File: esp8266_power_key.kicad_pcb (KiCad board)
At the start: 2 copper layers, 25 parts, among them P1 CONN_01X06, P2 CONN_01X06, Q1 Q_PMOS_GDS, Q2 Q_PMOS_GDS, Q3 BC849, Q4 BC849, U1 ESP-01v090, U2 LP2988AIMX-3.3/NOPB

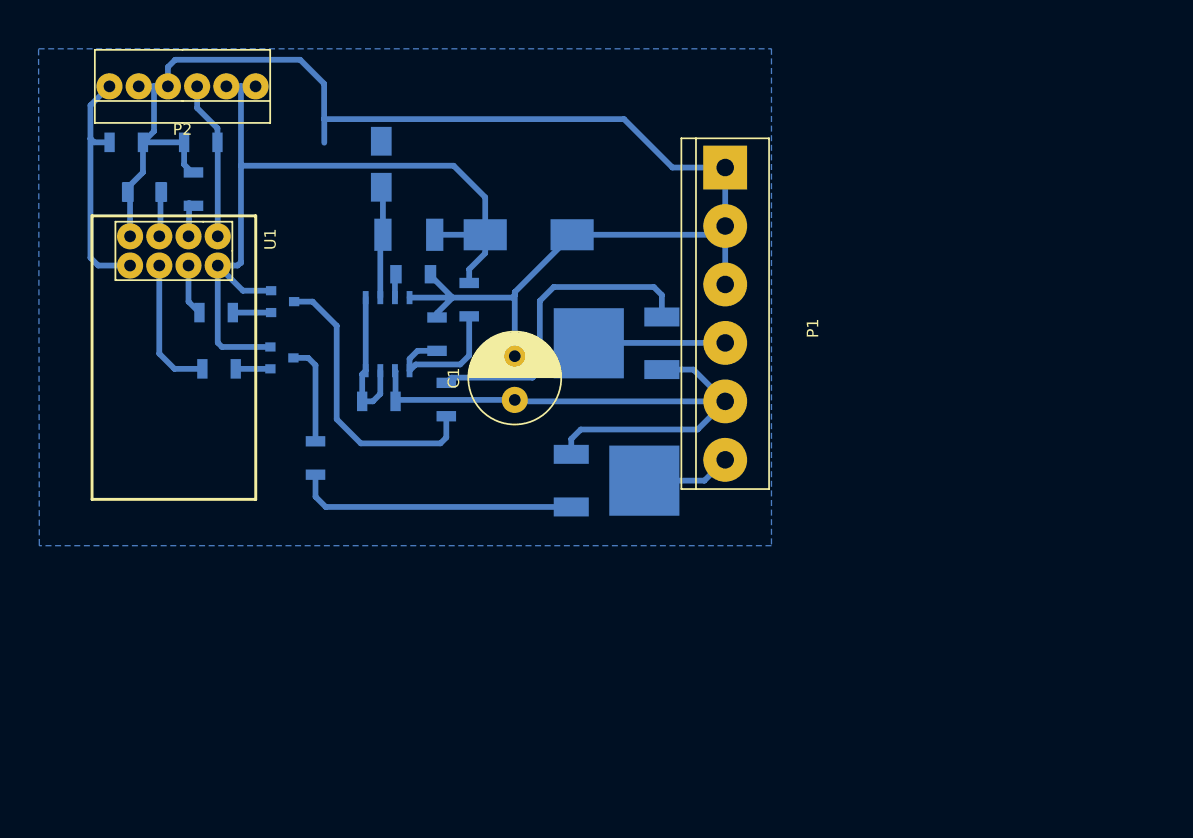
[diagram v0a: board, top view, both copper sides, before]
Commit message: 4 channel version
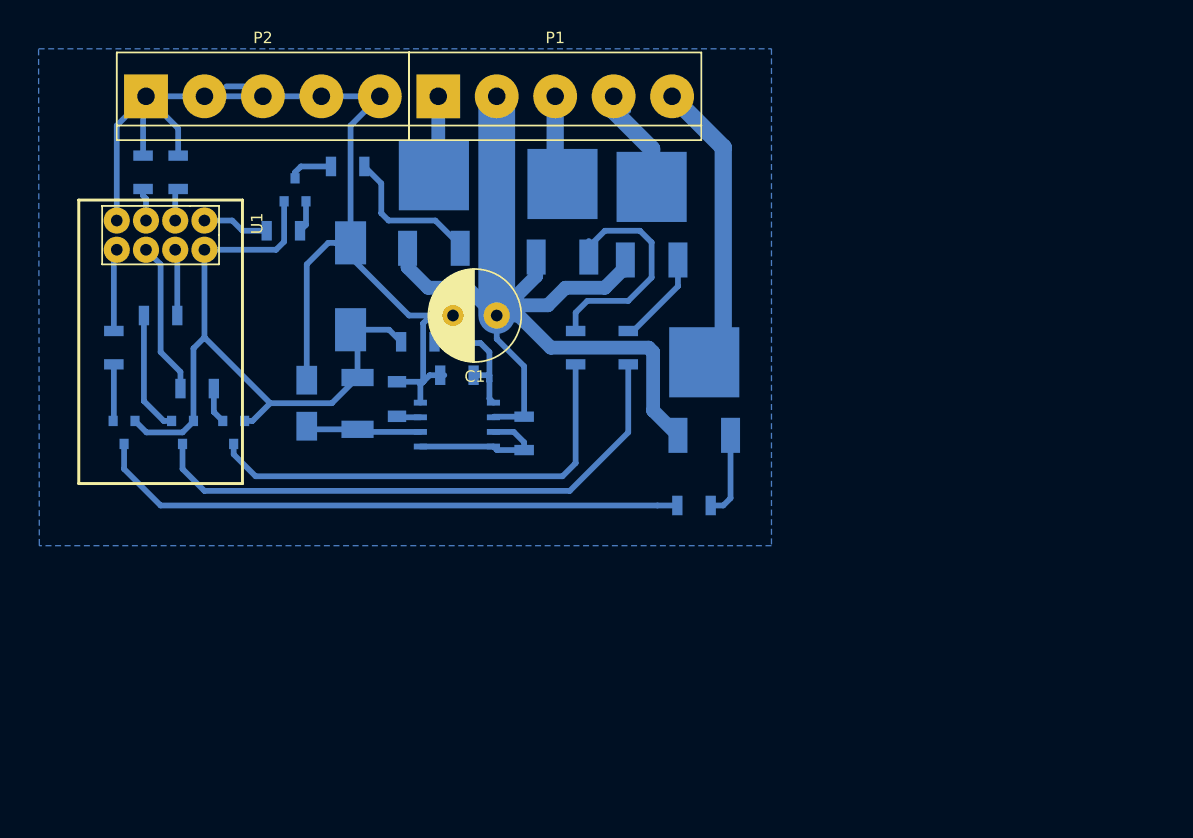
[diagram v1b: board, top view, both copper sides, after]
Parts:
- removed R1, R8: R, Resistors_SMD:R_1206
- removed the R2 at (29.0, 33.7)
- removed the R2 at (29.1, 33.7)
- added Q5: BC849, TO_SOT_Packages_SMD:SOT-23, B.Cu at (27.3, 54.6)
- added Q6: BC849, TO_SOT_Packages_SMD:SOT-23, B.Cu at (42.2, 33.5)
- added Q7: Q_PMOS_GDS, TO_SOT_Packages_SMD:TO-252-2Lead, B.Cu at (77.7, 54.9)
- added Q8: Q_PMOS_GDS, TO_SOT_Packages_SMD:TO-252-2Lead, B.Cu at (54.2, 38.6)
- added R12: R, Resistors_SMD:R_1206, B.Cu at (26.4, 47.2)
- added R13: R, Resistors_SMD:R_1206, B.Cu at (41.1, 37.1)
- added R14: R, Resistors_SMD:R_1206, B.Cu at (76.8, 61.0)
- added R15: R, Resistors_SMD:R_1206, B.Cu at (46.7, 31.5)
- added R2: R, Resistors_SMD:R_1206, B.Cu at (29.0, 32.0)
- P1: value CONN_01X06 -> CONN_01X05; footprint Connect:bornier6 -> Connect:bornier5
- P2: value CONN_01X06 -> CONN_01X05; footprint Connect:PINHEAD1-6 -> Connect:bornier5
- moved R4 24.6 mm to (66.5, 47.2), turned to 90 degrees
- moved P1 24.0 mm to (64.8, 25.4), turned to 0 degrees
- moved D1 21.8 mm to (43.2, 52.1)
- moved Q1 19.4 mm to (65.4, 39.4), turned to 180 degrees
- moved R5 16.4 mm to (71.1, 47.2)
- moved C2 16.1 mm to (47.0, 41.9), turned to 270 degrees
- moved L1 15.3 mm to (47.6, 52.1), turned to 270 degrees
- moved Q4 14.3 mm to (32.4, 54.6), turned to 270 degrees
- moved R6 12.9 mm to (62.1, 54.7), turned to 90 degrees
- moved C3 10.9 mm to (51.0, 51.7), turned to 90 degrees
- moved U2 9.90 mm to (56.2, 53.9), turned to 90 degrees
- moved Q3 7.71 mm to (36.8, 54.6), turned to 270 degrees
- moved C1 7.50 mm to (59.7, 44.5), turned to 180 degrees
- moved Q2 7.29 mm to (73.2, 39.6), turned to 180 degrees
- moved P2 7.04 mm to (39.4, 25.4), turned to 0 degrees
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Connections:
- P1 pad 1: GND -> Net-(P1-Pad1)
- P1 pad 2: GND -> Net-(C1-Pad1)
- P1 pad 3: GND -> Net-(P1-Pad3)
- P1 pad 5: Net-(C1-Pad1) -> Net-(P1-Pad5)
- P2 pad 1: Net-(C2-Pad2) -> GND
- P2 pad 2: Net-(C2-Pad2) -> GND
- P2 pad 3: Net-(P2-Pad3) -> GND
- Q1 pad 2: Net-(P1-Pad6) -> Net-(P1-Pad3)
- U1 pad 1: Net-(P2-Pad3) -> Net-(R13-Pad1)
- U1 pad 8: Net-(P2-Pad6) -> Net-(R12-Pad1)
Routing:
- net Net-(Q5-Pad3): track 0.00 -> 51.6 mm
- net Net-(C1-Pad1): track 55.9 -> 90.3 mm
- net Net-(Q3-Pad3): track 8.80 -> 40.5 mm
- net GND: track 131.6 -> 104.3 mm
- net Net-(P1-Pad5): track 0.00 -> 26.3 mm
- net Net-(Q4-Pad3): track 25.2 -> 49.7 mm
- net Net-(P2-Pad6): track 21.3 -> 0.00 mm
- net Net-(Q2-Pad1): track 27.9 -> 8.21 mm
- net Net-(Q8-Pad1): track 0.00 -> 14.6 mm
- net Net-(P2-Pad3): track 13.8 -> 0.00 mm
- net Net-(C2-Pad2): track 71.8 -> 60.6 mm
- net Net-(P1-Pad3): track 0.00 -> 8.78 mm
- net Net-(P1-Pad1): track 0.00 -> 8.09 mm
- net Net-(P1-Pad6): track 7.78 -> 0.00 mm
- net Net-(Q7-Pad1): track 0.00 -> 7.45 mm
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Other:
- net class pwr added: clearance 0.2, trace_width 1.5, via_dia 0.6, via_drill 0.4

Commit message: moved corners
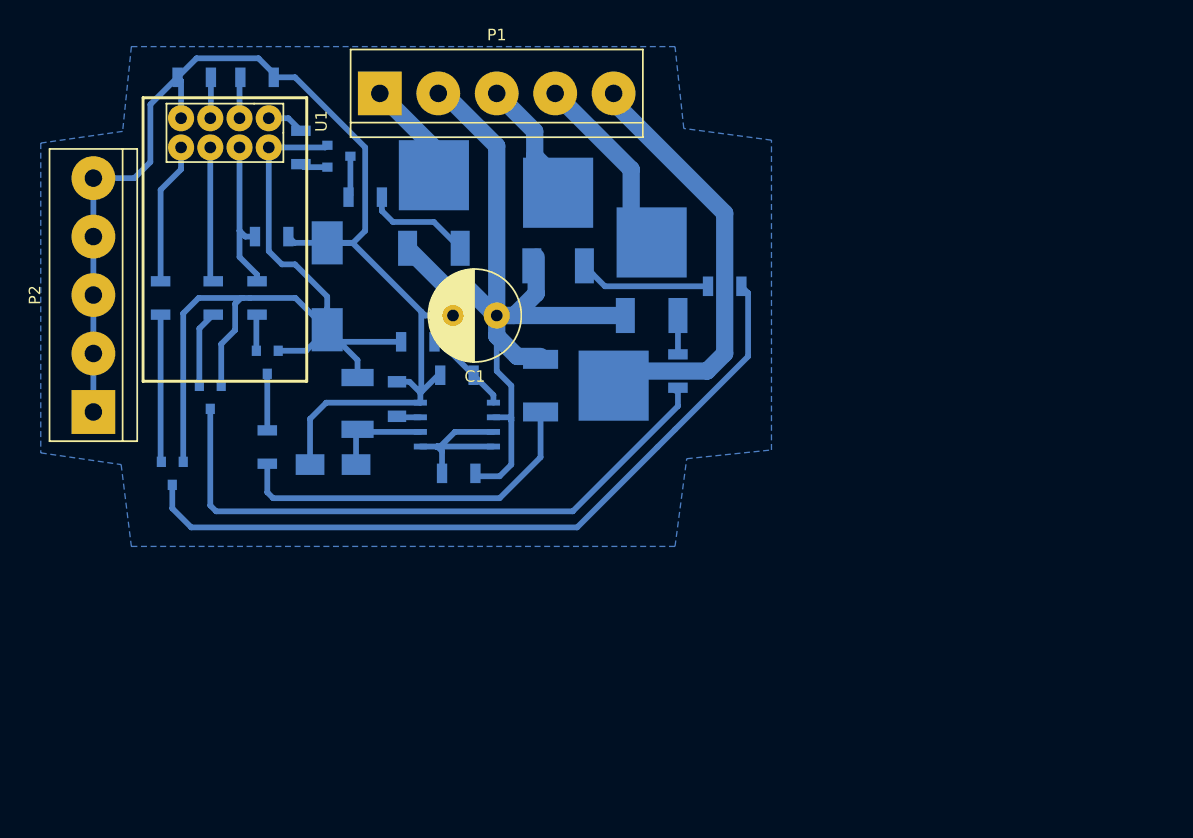
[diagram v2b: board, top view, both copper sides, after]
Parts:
- added R1: R, Resistors_SMD:R_1206, B.Cu at (40.1, 37.6)
- moved R14 37.4 mm to (39.8, 55.9), turned to 270 degrees
- moved P2 22.7 mm to (24.6, 42.7), turned to 90 degrees
- moved Q7 14.9 mm to (63.5, 50.5), turned to 90 degrees
- moved R4 14.0 mm to (79.5, 41.9), turned to 180 degrees
- moved R3 10.7 mm to (38.9, 23.7), turned to 0 degrees
- moved U1 10.5 mm to (39.9, 27.3)
- moved R9 9.44 mm to (38.9, 42.9), turned to 270 degrees
- moved R2 9.38 mm to (33.4, 23.7), turned to 180 degrees
- moved R13 7.40 mm to (42.7, 29.8), turned to 270 degrees
- moved Q3 6.76 mm to (39.8, 48.5)
- moved R6 6.66 mm to (56.4, 58.2), turned to 0 degrees
- moved R12 5.93 mm to (30.5, 42.9)
- moved D1 5.80 mm to (45.5, 57.4), turned to 180 degrees
- moved Q5 5.50 mm to (31.5, 58.2)
- moved P1 5.09 mm to (59.7, 25.1)
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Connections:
- R14 pad 1: Net-(Q5-Pad3) -> Net-(Q3-Pad3)
- R4 pad 1: Net-(Q3-Pad3) -> Net-(Q5-Pad3)
- R9 pad 1: Net-(R9-Pad1) -> Net-(R1-Pad2)
- U1 pad 4: Net-(R10-Pad1) -> Net-(R1-Pad2)
- U1 pad 6: Net-(R9-Pad1) -> Net-(R10-Pad1)
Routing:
- net Net-(Q3-Pad3): track 40.5 -> 4.92 mm
- net Net-(Q7-Pad1): track 7.45 -> 31.9 mm
- net Net-(C2-Pad2): track 60.6 -> 78.4 mm
- net Net-(C1-Pad1): track 90.3 -> 74.2 mm
- net Net-(P1-Pad5): track 26.3 -> 42.2 mm
- net Net-(R1-Pad2): track 0.00 -> 14.1 mm
- net Net-(Q5-Pad3): track 51.6 -> 65.3 mm
- net Net-(R9-Pad1): track 13.7 -> 0.00 mm
- net GND: track 104.3 -> 113.2 mm
- net Net-(Q1-Pad1): track 21.3 -> 12.6 mm
- net Net-(Q5-Pad1): track 4.94 -> 12.8 mm
- net Net-(R10-Pad1): track 5.79 -> 11.7 mm
- net Net-(Q4-Pad3): track 49.7 -> 55.0 mm
- net Net-(Q8-Pad1): track 14.6 -> 9.35 mm
- net Net-(R12-Pad1): track 7.16 -> 12.4 mm
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
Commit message: Rev 2.0
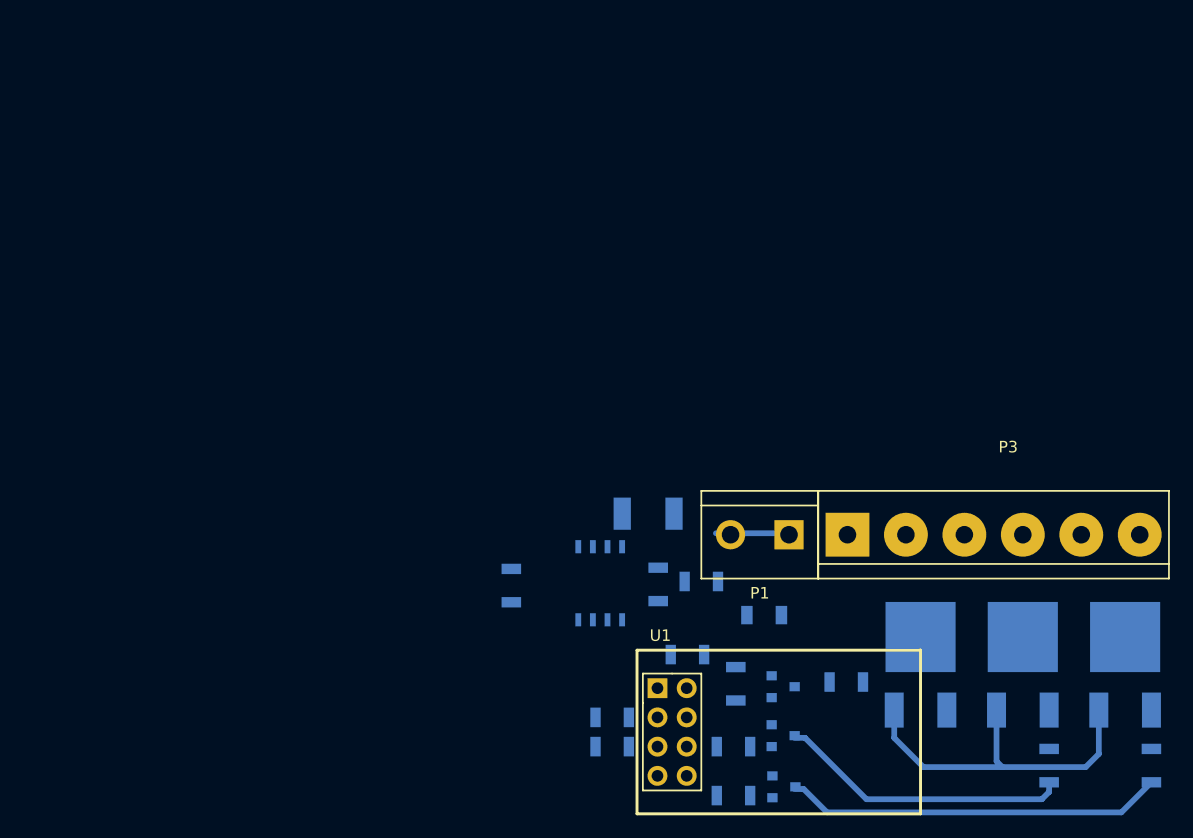
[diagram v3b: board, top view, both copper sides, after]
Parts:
- removed C1: CP, Capacitors_ThroughHole:C_Radial_D8_L13_P3.8
- removed C2: CP, Capacitors_Tantalum_SMD:Tantalum_Case-D_EIA-7343-31_Hand
- removed D1: D, Diodes_SMD:SMA_Standard
- removed P2: CONN_01X05, Connect:bornier5
- removed Q7, Q8: Q_PMOS_GDS, TO_SOT_Packages_SMD:TO-252-2Lead
- removed R13, R14, R15: R, Resistors_SMD:R_1206
- added P3: CONN_01X06, Connect:bornier6, F.Cu at (102.9, 63.5)
- added R8: R, Resistors_SMD:R_1206, B.Cu at (80.5, 76.5)
- P1: value CONN_01X05 -> CONN_01X02; footprint Connect:bornier5 -> Connect:bornier2
- Q1, Q2: value Q_PMOS_GDS -> Q_NMOS_GDS
- Q3: value BC849 -> Q_NMOS_GDS; footprint TO_SOT_Packages_SMD:SOT-23 -> TO_SOT_Packages_SMD:TO-252-2Lead
- moved R9 79.9 mm to (107.7, 83.6)
- moved R2 68.6 mm to (69.7, 81.9)
- moved R12 68.3 mm to (90.1, 76.3), turned to 180 degrees
- moved Q3 64.3 mm to (96.5, 78.7), turned to 180 degrees
- moved R3 63.6 mm to (69.7, 79.4), turned to 180 degrees
- moved Q1 62.6 mm to (114.3, 78.7)
- moved R10 62.6 mm to (80.3, 86.2), turned to 180 degrees
- moved Q4 60.3 mm to (84.6, 85.4), turned to 0 degrees
- moved Q6 60.1 mm to (84.6, 76.7)
- moved U1 60.0 mm to (73.7, 76.8), turned to 0 degrees
- moved Q5 57.8 mm to (84.6, 81.0), turned to 0 degrees
- moved R4 55.8 mm to (116.6, 83.6), turned to 270 degrees
- moved R1 51.2 mm to (76.3, 73.9)
- moved Q2 47.1 mm to (105.4, 78.7)
- moved P1 44.6 mm to (82.5, 63.5), turned to 180 degrees
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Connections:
- L1 pad 1: Net-(C2-Pad2) -> +3V3
- P1 pad 1: Net-(P1-Pad1) -> +36V
- P1 pad 2: Net-(C1-Pad1) -> GND
- Q1 pad 2: Net-(P1-Pad3) -> Net-(P3-Pad5)
- Q1 pad 3: Net-(C1-Pad1) -> +36V
- Q2 pad 2: Net-(P1-Pad4) -> Net-(P3-Pad3)
- Q2 pad 3: Net-(C1-Pad1) -> +36V
- Q3 pad 2: Net-(C2-Pad2) -> Net-(P3-Pad1)
- Q3 pad 3: Net-(Q3-Pad3) -> +36V
- Q4 pad 2: Net-(C2-Pad2) -> GND
- Q5 pad 2: Net-(C2-Pad2) -> GND
- Q6 pad 2: Net-(C2-Pad2) -> GND
- R1 pad 1: GND -> Net-(Q4-Pad1)
- R10 pad 1: Net-(R10-Pad1) -> Net-(Q6-Pad1)
- R10 pad 2: Net-(Q4-Pad1) -> Net-(R10-Pad2)
- R12 pad 1: Net-(R12-Pad1) -> Net-(Q3-Pad1)
- R12 pad 2: Net-(Q5-Pad1) -> Net-(Q6-Pad3)
- R4 pad 1: Net-(Q5-Pad3) -> Net-(Q1-Pad1)
- R4 pad 2: Net-(Q1-Pad1) -> Net-(Q4-Pad3)
- R5 pad 1: Net-(Q4-Pad3) -> Net-(Q5-Pad1)
- R5 pad 2: Net-(Q2-Pad1) -> Net-(R5-Pad2)
- R6 pad 2: Net-(C1-Pad1) -> +36V
- R7 pad 2: Net-(C2-Pad2) -> +3V3
- R9 pad 1: Net-(R1-Pad2) -> Net-(Q2-Pad1)
- R9 pad 2: Net-(Q3-Pad1) -> Net-(Q5-Pad3)
- U1 pad 1: Net-(R13-Pad1) -> Net-(R1-Pad2)
- U1 pad 2: Net-(C2-Pad2) -> GND
- U1 pad 4: Net-(R1-Pad2) -> Net-(R8-Pad2)
- U1 pad 6: Net-(R10-Pad1) -> Net-(R5-Pad2)
- U1 pad 7: GND -> +3V3
- U1 pad 8: Net-(R12-Pad1) -> Net-(R10-Pad2)
- U2 pad 6: Net-(C1-Pad1) -> +36V
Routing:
- net GND: track 113.2 -> 0.00 mm
- net Net-(C2-Pad2): track 78.4 -> 0.00 mm
- net Net-(C1-Pad1): track 74.2 -> 0.00 mm
- net Net-(P1-Pad5): track 42.2 -> 0.00 mm
- net Net-(Q5-Pad3): track 65.3 -> 25.4 mm
- net +36V: track 0.00 -> 36.8 mm
- net Net-(Q7-Pad1): track 31.9 -> 0.00 mm
- net Net-(Q4-Pad3): track 55.0 -> 32.9 mm
- net Net-(P1-Pad4): track 16.4 -> 0.00 mm
- net Net-(R6-Pad1): track 14.4 -> 0.00 mm
- net Net-(R1-Pad2): track 14.1 -> 0.00 mm
- net Net-(Q5-Pad1): track 12.8 -> 0.00 mm
- net Net-(Q1-Pad1): track 12.6 -> 0.00 mm
- net Net-(R12-Pad1): track 12.4 -> 0.00 mm
- net Net-(R10-Pad1): track 11.7 -> 0.00 mm
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- removed copper zone on B.Cu, net GND
